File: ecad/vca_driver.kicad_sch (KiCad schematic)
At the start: 17 parts, among them Q2 BD140, Q4 BD139, U3 OPA2277

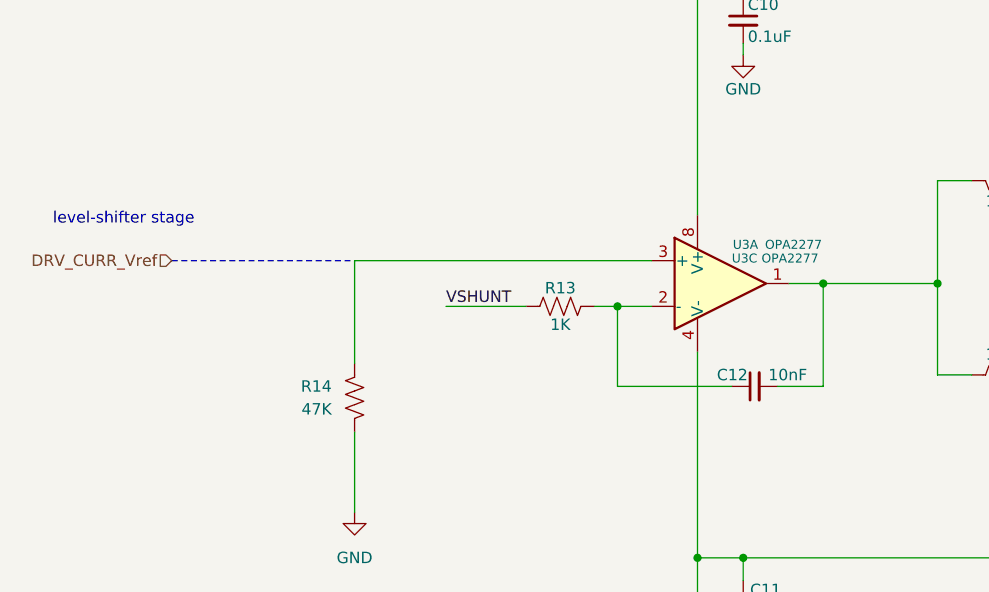
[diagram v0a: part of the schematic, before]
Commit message: vca sims
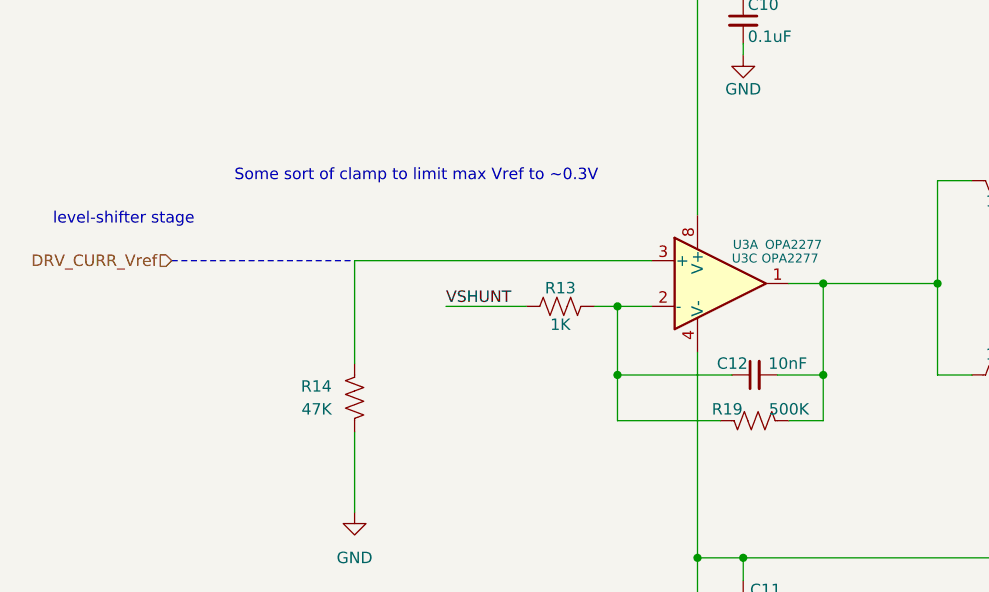
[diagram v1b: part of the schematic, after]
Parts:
- added R19: 500K, symbol Device:R_US
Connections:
- net at C12.1, R13.2, U3.2 (-): now also R19.1
- net at C12.2, R11.2, R12.2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: now also R19.2
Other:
- note added: "Some sort of clamp to limit max Vref to ~0.3V"
- moved on the sheet: C12
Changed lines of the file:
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@@
+		)
+	)
+	(text "Some sort of clamp to limit max Vref to ~0.3V"
+		(exclude_from_sim no)
+		(at 77.978 82.042 0)
+		(effects
+			(font
+				(size 1.27 1.27)
+			)
 		)
 	)
@@
 	)
 	(junction
+		(at 100.33 104.14)
+		(diameter 0)
+		(color 0 0 0 0)
+	)
+	(junction
 		(at 100.33 96.52)
 		(diameter 0)
@@
 	(junction
 		(at 148.59 124.46)
+		(diameter 0)
+		(color 0 0 0 0)
+	)
+	(junction
+		(at 123.19 104.14)
 		(diameter 0)
 		(color 0 0 0 0)
@@
 	(wire
 		(pts
+			(xy 100.33 104.14) (xy 100.33 96.52)
+		)
+		(stroke
+			(width 0)
+			(type default)
+		)
+	)
+	(wire
+		(pts
 			(xy 97.79 96.52) (xy 100.33 96.52)
 		)
@@
 	(wire
 		(pts
+			(xy 111.76 109.22) (xy 100.33 109.22)
+		)
+		(stroke
+			(width 0)
+			(type default)
+		)
+	)
+	(wire
+		(pts
 			(xy 157.48 119.38) (xy 157.48 124.46)
 		)
@@
 	(wire
 		(pts
-			(xy 118.11 105.41) (xy 123.19 105.41)
+			(xy 118.11 104.14) (xy 123.19 104.14)
 		)
 		(stroke
@@
 	(wire
 		(pts
+			(xy 123.19 104.14) (xy 123.19 109.22)
+		)
+		(stroke
+			(width 0)
+			(type default)
+		)
+	)
+	(wire
+		(pts
 			(xy 135.89 82.55) (xy 139.7 82.55)
 		)
@@
 	(wire
 		(pts
+			(xy 119.38 109.22) (xy 123.19 109.22)
+		)
+		(stroke
+			(width 0)
+			(type default)
+		)
+	)
+	(wire
+		(pts
 			(xy 157.48 72.39) (xy 157.48 77.47)
 		)
@@
 	(wire
 		(pts
-			(xy 113.03 105.41) (xy 100.33 105.41)
+			(xy 113.03 104.14) (xy 100.33 104.14)
 		)
 		(stroke
@@
 	(wire
 		(pts
+			(xy 123.19 104.14) (xy 123.19 93.98)
+		)
+		(stroke
+			(width 0)
+			(type default)
+		)
+	)
+	(wire
+		(pts
 			(xy 147.32 67.31) (xy 147.32 68.58)
 		)
@@
 	(wire
 		(pts
-			(xy 100.33 105.41) (xy 100.33 96.52)
-		)
-		(stroke
-			(width 0)
-			(type default)
-		)
-	)
-	(wire
-		(pts
 			(xy 203.2 113.03) (xy 203.2 115.57)
 		)
@@
 	(wire
 		(pts
+			(xy 100.33 104.14) (xy 100.33 109.22)
+		)
+		(stroke
+			(width 0)
+			(type default)
+		)
+	)
+	(wire
+		(pts
 			(xy 71.12 91.44) (xy 104.14 91.44)
 		)
@@
 		(pts
 			(xy 135.89 93.98) (xy 135.89 82.55)
-		)
-		(stroke
-			(width 0)
-			(type default)
-		)
-	)
-	(wire
-		(pts
-			(xy 123.19 105.41) (xy 123.19 93.98)
 		)
 		(stroke
@@
 	(symbol
 		(lib_id "Device:C_Small")
-		(at 115.57 105.41 90)
+		(at 115.57 104.14 90)
 		(unit 1)
 		(body_style 1)
@@
 		(dnp no)
 		(property "Reference" "C12"
-			(at 114.808 104.14 90)
+			(at 114.808 102.87 90)
 			(show_name no)
 			(do_not_autoplace no)
@@
 		)
 		(property "Value" "10nF"
-			(at 121.412 104.14 90)
+			(at 121.412 102.87 90)
 			(show_name no)
 			(do_not_autoplace no)
@@
 		)
 		(property "Footprint" ""
-			(at 115.57 105.41 0)
+			(at 115.57 104.14 0)
 			(hide yes)
 			(show_name no)
@@
 		)
 		(property "Datasheet" ""
-			(at 115.57 105.41 0)
+			(at 115.57 104.14 0)
 			(hide yes)
 			(show_name no)
@@
 		)
 		(property "Description" "Unpolarized capacitor, small symbol"
-			(at 115.57 105.41 0)
+			(at 115.57 104.14 0)
 			(hide yes)
 			(show_name no)
@@
 					(unit 1)
 				)
+			)
+		)
+	)
+	(symbol
+		(lib_id "Device:R_US")
+		(at 115.57 109.22 90)
+		(mirror x)
+		(unit 1)
+		(body_style 1)
+		(exclude_from_sim no)
+		(in_bom yes)
+		(on_board yes)
+		(in_pos_files yes)
+		(dnp no)
+		(property "Reference" "R19"
+			(at 112.522 107.95 90)
+			(show_name no)
+			(do_not_autoplace no)
+			(effects
+				(font
+					(size 1.27 1.27)
+				)
+			)
+		)
+		(property "Value" "500K"
+			(at 119.38 107.95 90)
+			(show_name no)
+			(do_not_autoplace no)
+			(effects
+				(font
+					(size 1.27 1.27)
+				)
+			)
+		)
+		(property "Footprint" ""
+			(at 115.824 110.236 90)
+			(hide yes)
+			(show_name no)
+			(do_not_autoplace no)
+			(effects
+				(font
+					(size 1.27 1.27)
+				)
+			)
+		)
+		(property "Datasheet" ""
+			(at 115.57 109.22 0)
+			(hide yes)
+			(show_name no)
+			(do_not_autoplace no)
+			(effects
+				(font
+					(size 1.27 1.27)
+				)
+			)
+		)
+		(property "Description" "Resistor, US symbol"
+			(at 115.57 109.22 0)
+			(hide yes)
+			(show_name no)
+			(do_not_autoplace no)
+			(effects
+				(font
+					(size 1.27 1.27)
+				)
+			)
+		)
+		(pin "2"
+		)
+		(pin "1"
+		)
+		(instances
+			(project "afm"
+				(path "/62de9aa8-4539-4ecb-8acc-2c7a46b3005b/152e488a-5c59-4955-a770-fd5dc463781b"
+					(reference "R19")
+					(unit 1)
+				)
